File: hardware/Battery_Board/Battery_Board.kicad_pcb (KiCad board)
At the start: 2 copper layers, 83 x 83 mm, 28 parts, among them J1 Source, J3 Battery, P1 USB_C_Plug_USB2.0, Q1 DMG3415U-7, SW3 ON, U4 TP4056

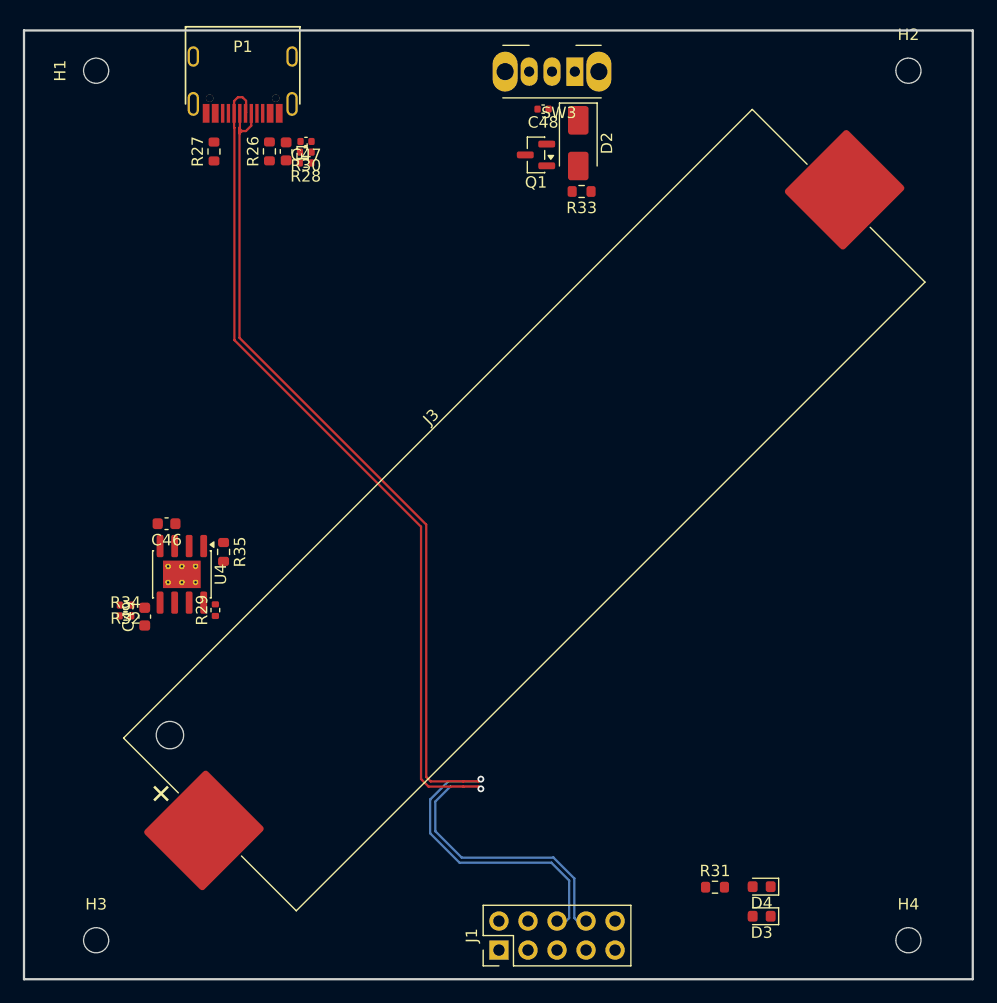
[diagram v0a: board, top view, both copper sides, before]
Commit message: feat(Hw):PCB_PwnSat_And_Battery_Updated
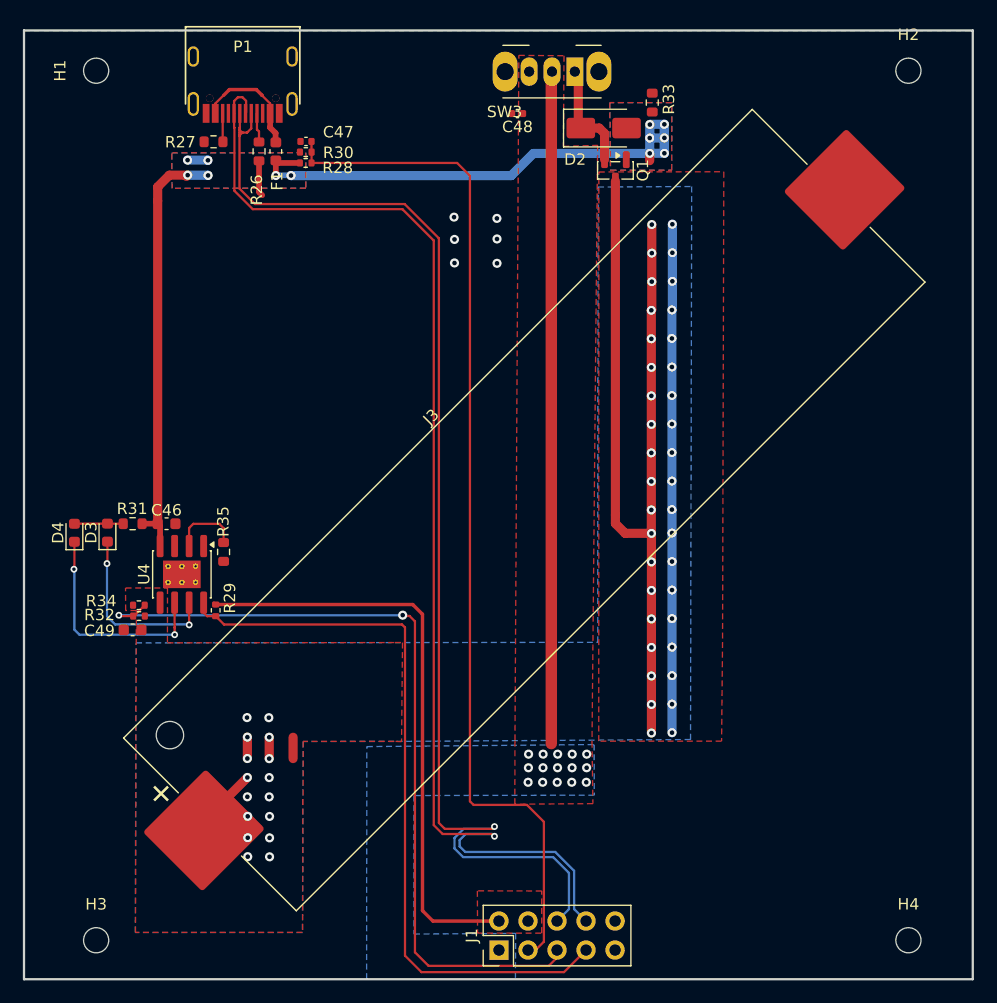
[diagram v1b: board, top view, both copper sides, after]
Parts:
- moved D4 67.6 mm to (67.0, 146.4), turned to 90 degrees
- moved D3 66.3 mm to (69.9, 146.4), turned to 90 degrees
- moved R31 60.1 mm to (72.1, 145.6), turned to 180 degrees
- moved R33 9.93 mm to (117.6, 108.8), turned to 90 degrees
- moved Q1 7.08 mm to (114.3, 114.7), turned to -90 degrees
- moved D2 2.58 mm to (113.3, 111.0), turned to 0 degrees
- moved C48 2.27 mm to (105.8, 109.7)
- moved C49 1.57 mm to (72.1, 154.9), turned to 180 degrees
- moved R32 1.51 mm to (72.7, 153.7)
- moved R34 1.49 mm to (72.7, 152.8), turned to 180 degrees
- moved R26 0.91 mm to (83.2, 113.0)
- moved F1 0.90 mm to (84.6, 113.0)
- moved R27 0.85 mm to (79.2, 112.2), turned to 0 degrees
- turned R29 to -90 degrees
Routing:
- net +BATT: track 0.00 -> 134.2 mm, vias 0 -> 54
- net /Batt_Connector/USB_DET: track 0.00 -> 90.3 mm
- net VBUS: track 0.00 -> 88.7 mm, vias 0 -> 12
- net /Batt_Connector/Battery: track 0.00 -> 71.6 mm, vias 0 -> 2
- net /Batt_Connector/Enable: track 0.00 -> 65.0 mm
- net VCC: track 0.00 -> 59.2 mm, vias 0 -> 15
- net +3.3V: track 0.00 -> 51.7 mm
- net Net-(D4-K): track 0.00 -> 19.5 mm, vias 0 -> 2
- net Net-(D3-K): track 0.00 -> 16.0 mm, vias 0 -> 2
- net Net-(F1-Pad1): track 0.00 -> 10.3 mm
- net Net-(D2-K): track 0.00 -> 9.72 mm
- net /Batt_Connector/2_DN: track 99.2 -> 105.7 mm
- net Net-(U4-PROG): track 0.00 -> 6.16 mm
- net /Batt_Connector/2_DP: track 99.8 -> 106.0 mm
- net Net-(D3-A): track 0.00 -> 4.28 mm
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- added copper zone on F.Cu, net +3.3V
- added copper zone on B.Cu, net +BATT
- added copper zone on F.Cu, net +BATT
- added copper zone on B.Cu, net GND
- added copper zone on F.Cu, net GND
- added copper zone on B.Cu, net VBUS
- added copper zone on F.Cu, net VBUS
- added copper zone on B.Cu, net VCC
- added copper zone on F.Cu, net VCC
